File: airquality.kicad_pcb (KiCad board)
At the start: 2 copper layers, 99.9 x 99.9 mm, 26 parts, among them J1 MHZ19, J2 Conn_02x10_Odd_Even, J3 Conn_02x10_Odd_Even, J4 Conn_01x04_Female, J5 Conn_01x04_Male, J6 Conn_01x04_Female, J7 Conn_01x04_Male, J8 Conn_01x04_Male, U1 DS18B20, U2 PMS7003, U3 RFM95W-868S2, U4 DS18B20, U5 DS18B20

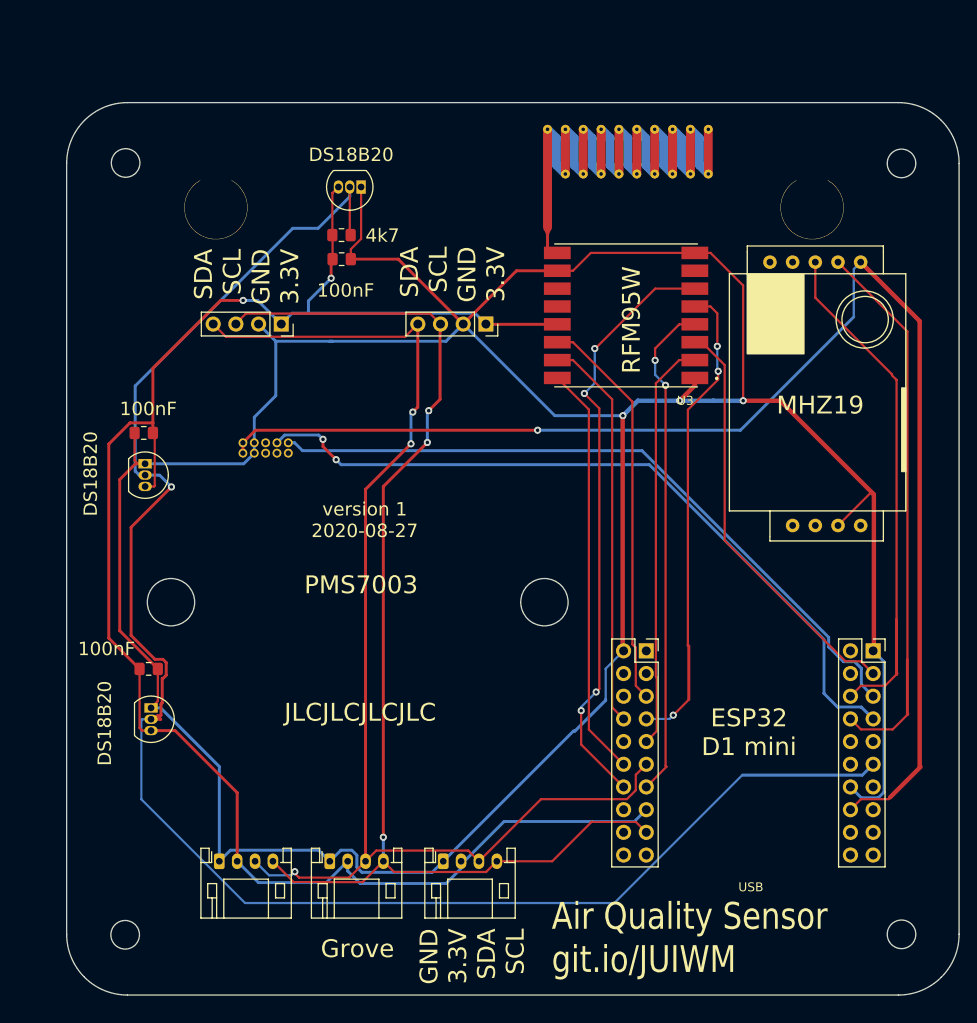
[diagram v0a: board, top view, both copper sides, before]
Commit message: rev2
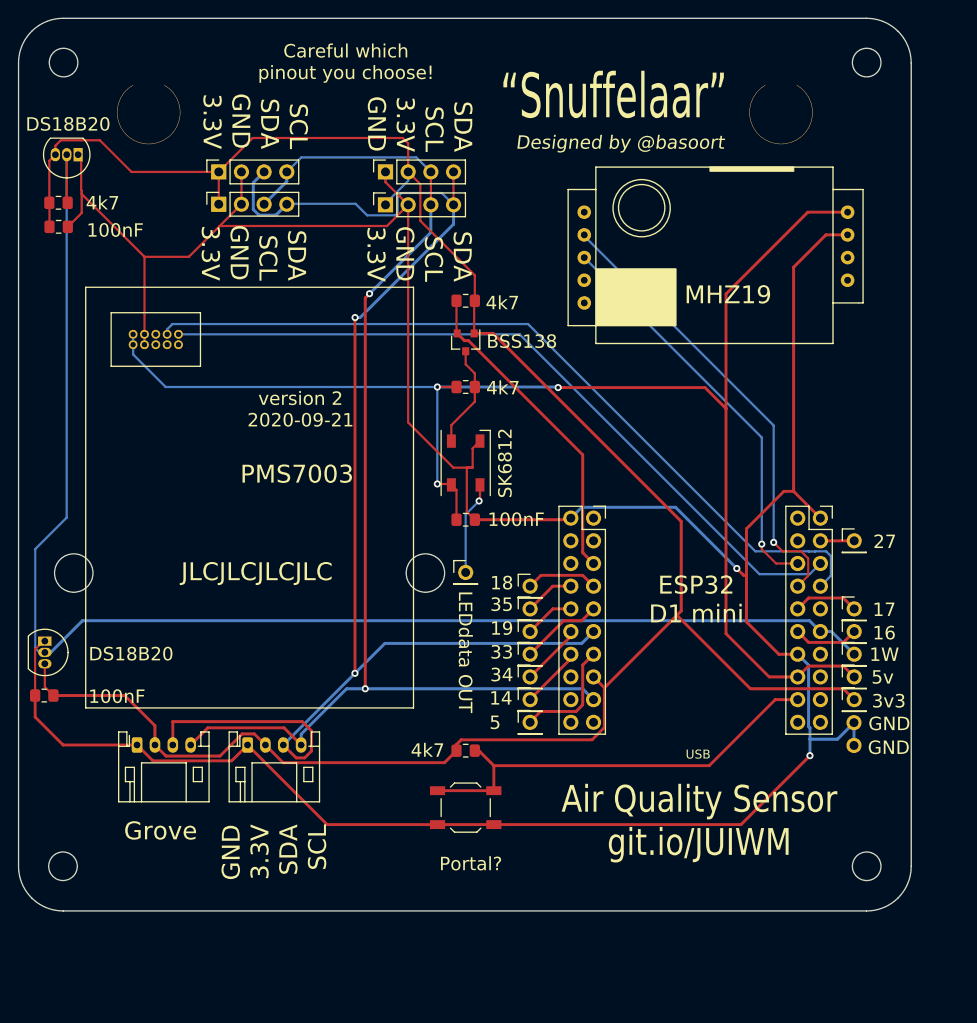
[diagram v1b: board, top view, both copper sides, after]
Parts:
- removed AE1: Antenna, RF_Antenna:Texas_SWRA416_868MHz_915MHz
- removed C3: 100nF, Capacitor_SMD:C_0805_2012Metric_Pad1.15x1.40mm_HandSolder
- removed G*** (x2): LOGO, parts_models:keyhole
- removed REF** (x2): MountingHole_5.3mm_M5, MountingHole:MountingHole_5.3mm_M5
- removed REF** (x4): MountingHole_3.2mm_M3, MountingHole:MountingHole_3.2mm_M3
- removed the U3 at (163.6, 80.3)
- removed U5: DS18B20, Package_TO_SOT_THT:TO-92_Inline
- added C1: 100nF, Capacitor_SMD:C_0805_2012Metric_Pad1.15x1.40mm_HandSolder, F.Cu at (145.7, 103.2)
- added D1: SK6812, LED_SMD:LED_SK6812_PLCC4_5.0x5.0mm_P3.2mm, F.Cu at (145.7, 96.8)
- added H1: MountingHole, MountingHole:MountingHole_4.3mm_M4, F.Cu at (101.8, 109.2)
- added H2: MountingHole, MountingHole:MountingHole_4.3mm_M4, F.Cu at (141.2, 109.2)
- added H3: MountingHole, parts_models:keyhole, F.Cu at (175.3, 55.9)
- added H4: MountingHole, parts_models:keyhole, F.Cu at (104.5, 55.9)
- added H5: MountingHole, MountingHole:MountingHole_3.2mm_M3, F.Cu at (100.6, 52.0)
- added H6: MountingHole, MountingHole:MountingHole_3.2mm_M3, F.Cu at (190.6, 142.0)
- added H7: MountingHole, MountingHole:MountingHole_3.2mm_M3, F.Cu at (190.6, 52.0)
- added H8: MountingHole, MountingHole:MountingHole_3.2mm_M3, F.Cu at (100.6, 142.0)
- added J10: Conn_01x01_Male, Connector_PinHeader_2.54mm:PinHeader_1x01_P2.54mm_Vertical, F.Cu at (152.9, 120.8)
- added J11: Conn_01x01_Male, Connector_PinHeader_2.54mm:PinHeader_1x01_P2.54mm_Vertical, F.Cu at (152.9, 115.7)
- added J13: Conn_01x01_Male, Connector_PinHeader_2.54mm:PinHeader_1x01_P2.54mm_Vertical, F.Cu at (189.2, 123.3)
- added J14: Conn_01x01_Male, Connector_PinHeader_2.54mm:PinHeader_1x01_P2.54mm_Vertical, F.Cu at (189.1, 125.9)
- added J15: Conn_01x01_Male, Connector_PinHeader_2.54mm:PinHeader_1x01_P2.54mm_Vertical, F.Cu at (189.1, 128.5)
- added J16: Conn_01x01_Male, Connector_PinHeader_2.54mm:PinHeader_1x01_P2.54mm_Vertical, F.Cu at (189.2, 120.8)
- added J2: Conn_01x01_Male, Connector_PinHeader_2.54mm:PinHeader_1x01_P2.54mm_Vertical, F.Cu at (189.2, 105.5)
- added J22: Conn_01x01_Male, Connector_PinHeader_2.54mm:PinHeader_1x01_P2.54mm_Vertical, F.Cu at (189.2, 118.2)
- added J23: Conn_01x04_Female, Connector_PinSocket_2.54mm:PinSocket_1x04_P2.54mm_Vertical, F.Cu at (136.7, 64.2)
- added J24: Conn_01x04_Female, Connector_PinSocket_2.54mm:PinSocket_1x04_P2.54mm_Vertical, F.Cu at (118.0, 64.2)
- added J25: Conn_01x01_Male, Connector_PinHeader_2.54mm:PinHeader_1x01_P2.54mm_Vertical, F.Cu at (145.7, 109.1)
- added J3: Conn_01x01_Male, Connector_PinHeader_2.54mm:PinHeader_1x01_P2.54mm_Vertical, F.Cu at (189.2, 113.2)
- added J4: Conn_01x01_Male, Connector_PinHeader_2.54mm:PinHeader_1x01_P2.54mm_Vertical, F.Cu at (189.2, 115.7)
- added J5: Conn_01x01_Male, Connector_PinHeader_2.54mm:PinHeader_1x01_P2.54mm_Vertical, F.Cu at (152.9, 118.2)
- added J6: Conn_01x01_Male, Connector_PinHeader_2.54mm:PinHeader_1x01_P2.54mm_Vertical, F.Cu at (152.9, 125.9)
- added J7: Conn_01x01_Male, Connector_PinHeader_2.54mm:PinHeader_1x01_P2.54mm_Vertical, F.Cu at (152.9, 110.6)
- added J9: Conn_01x01_Male, Connector_PinHeader_2.54mm:PinHeader_1x01_P2.54mm_Vertical, F.Cu at (152.9, 113.2)
- added Q1: BSS138, Package_TO_SOT_SMD:SOT-23, F.Cu at (145.7, 83.3)
- added R1: 4k7, Resistor_SMD:R_0805_2012Metric_Pad1.15x1.40mm_HandSolder, F.Cu at (145.7, 78.7)
- added R2: 4k7, Resistor_SMD:R_0805_2012Metric_Pad1.15x1.40mm_HandSolder, F.Cu at (145.7, 129.0)
- added R3: 4k7, Resistor_SMD:R_0805_2012Metric_Pad1.15x1.40mm_HandSolder, F.Cu at (145.7, 88.3)
- added SW1: SW_Push, Button_Switch_SMD:SW_SPST_TL3342, F.Cu at (145.7, 135.4)
- J8: value Conn_01x04_Male -> Conn_01x01_Male; footprint Connector_JST:JST_PH_S4B-PH-K_1x04_P2.00mm_Horizontal -> Connector_PinHeader_2.54mm:PinHeader_1x01_P2.54mm_Vertical
- moved C5 31.9 mm to (100.1, 70.4)
- moved R4 31.9 mm to (100.1, 67.7)
- moved U2 31.9 mm to (102.3, 62.3)
- moved C6 31.4 mm to (98.5, 122.9)
- moved U3 22.8 mm to (98.6, 116.8)
- moved J8 20.5 mm to (152.9, 123.3)
- moved J17 19.5 mm to (159.0, 81.5), turned to 180 degrees
- moved J18 17.4 mm to (136.7, 67.9), turned to 90 degrees
- moved U1 17.3 mm to (121.5, 100.7)
- moved J1 16.0 mm to (160.0, 103.0)
- moved J12 16.0 mm to (185.4, 103.0)
- moved J20 15.9 mm to (108.9, 128.4)
- moved J21 15.9 mm to (121.2, 128.4)
- moved J19 15.1 mm to (118.0, 67.9), turned to 90 degrees
- renumbered C1 to C5, C2 to C6, J2 to J1, J3 to J12, J1 to J17, J4 to J18, J6 to J19, J5 to J20, J7 to J21, R1 to R4, U2 to U1, U1 to U2, U4 to U3
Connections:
- J1 pad 16: NC -> Net-(J1-Pad16)
- J1 pad 4: NC -> Net-(J1-Pad4)
- J17 pad 1: Net-(J1-Pad1) -> 5V
- J17 pad 3: 5V -> Net-(J17-Pad3)
- J8 pad 1: GND -> IO14
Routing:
- net IO14: track 67.8 -> 6.98 mm, vias 4 -> 0
- net IO15: track 0.00 -> 49.0 mm
- net 3.3V: track 194.5 -> 243.3 mm, vias 2 -> 0
- net IO18: track 53.2 -> 8.11 mm, vias 3 -> 0
- net IO5: track 56.1 -> 12.9 mm, vias 2 -> 0
- net IO27: track 46.8 -> 3.78 mm
- net IO34: track 46.3 -> 6.97 mm
- net IO35: track 44.3 -> 5.61 mm
- net IO19: track 46.0 -> 9.20 mm
- net GND: track 370.6 -> 337.7 mm, vias 3 -> 2
- net 1wire: track 188.7 -> 157.0 mm, vias 1 -> 0
- net I2C_SDA: track 138.9 -> 157.0 mm, vias 3 -> 2
- net 5V: track 151.0 -> 162.7 mm, vias 1 -> 3
- net Net-(D1-Pad2): track 0.00 -> 11.6 mm
- net IO22: track 56.3 -> 45.6 mm, vias 0 -> 1
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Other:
- outline, holes or cut-outs redrawn
- board text added: "14"
- board text added: "16"
- board text added: "17"
- board text added: "18"
- board text added: "19"
- board text added: "1W"
- board text added: "27"
- board text added: "33"
- board text added: "34"
- board text added: "35"
- board text added: "3v3"
- board text added: "5"
- board text added: "5v"
- board text added: "BSS138"
- board text added: "Careful which pinout you choose!"
- board text added: "Designed by @basoort"
- board text added: "GND"
- board text added: "LEDdata OUT"
- board text added: "Portal?"
- board text added: "SCL SDA GND 3.3V"
- board text added: "SDA SCL 3.3V GND"
- board text added: "SK6812"
- board text added: "version 2 2020-09-21"
- board text added: "“Snuffelaar”"
- board text removed: "RFM95W"
- board text removed: "version 1 2020-08-27"
